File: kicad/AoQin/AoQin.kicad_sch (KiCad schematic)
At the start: 15 parts, among them J1 Conn_02x03_Odd_Even, J10 Conn_02x03_Odd_Even, J11 Conn_02x03_Odd_Even, J12 Conn_02x03_Odd_Even, J14 Screw_Terminal_01x04, J15 Screw_Terminal_01x04, J16 Screw_Terminal_01x04, J2 Conn_02x03_Odd_Even, J3 Screw_Terminal_01x04, J4 Screw_Terminal_01x04, J5 Conn_02x03_Odd_Even, J6 Screw_Terminal_01x04, J8 Screw_Terminal_01x03, J9 Screw_Terminal_01x03

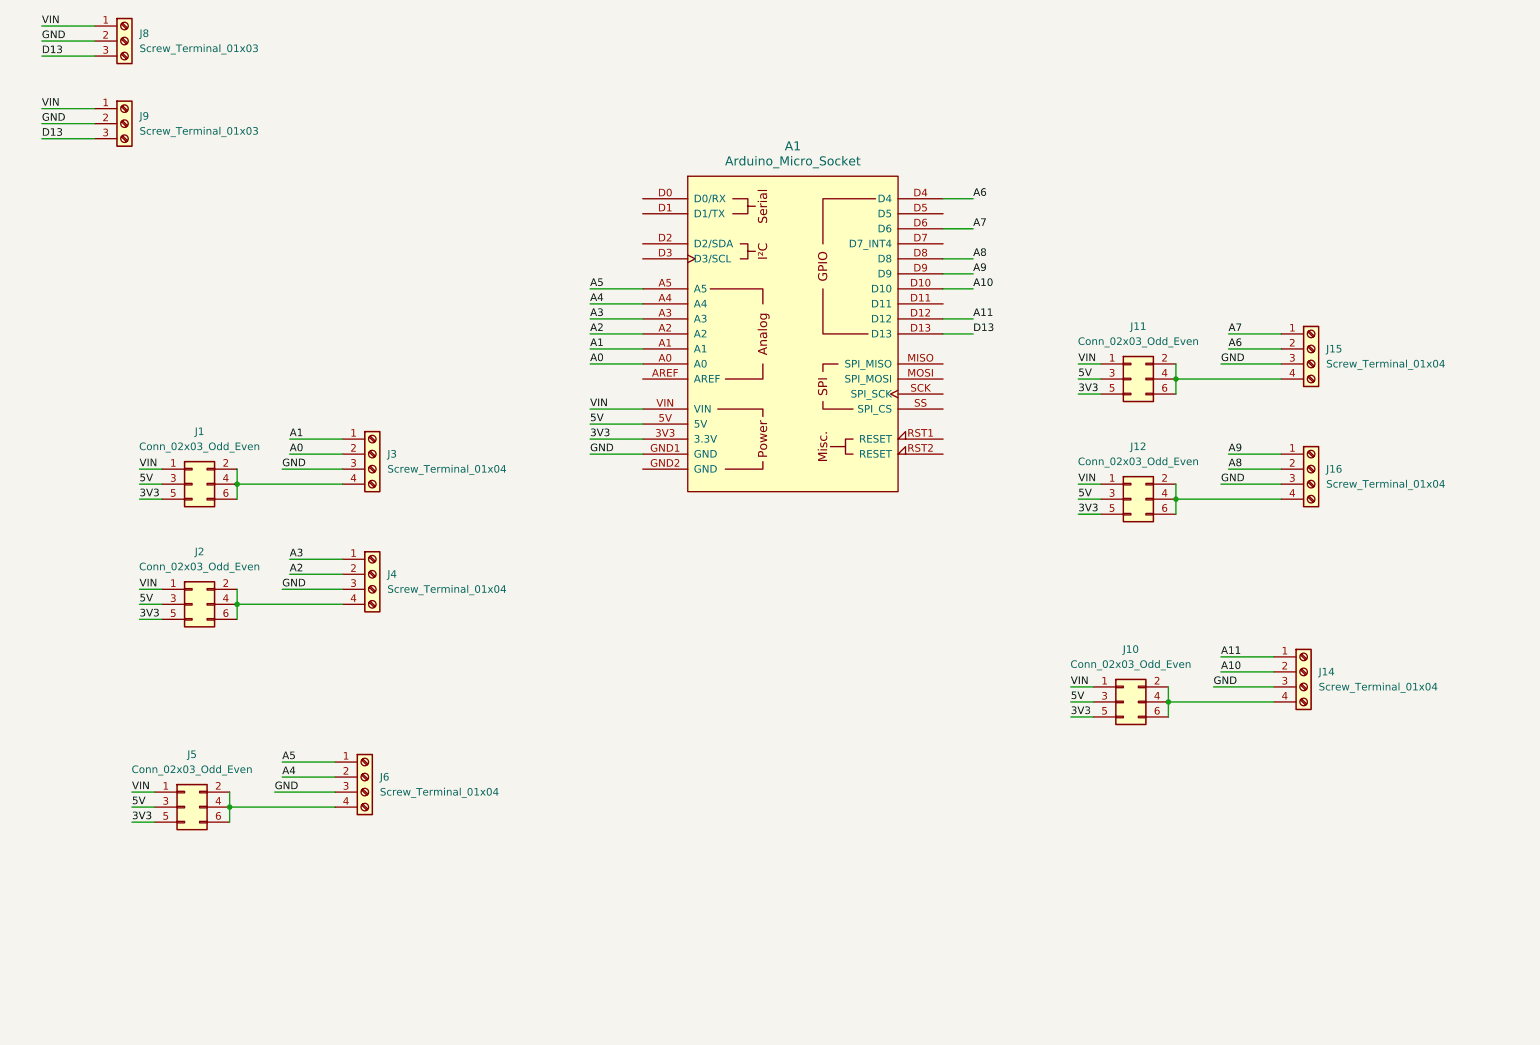
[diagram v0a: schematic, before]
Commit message: The Cave of Echoes
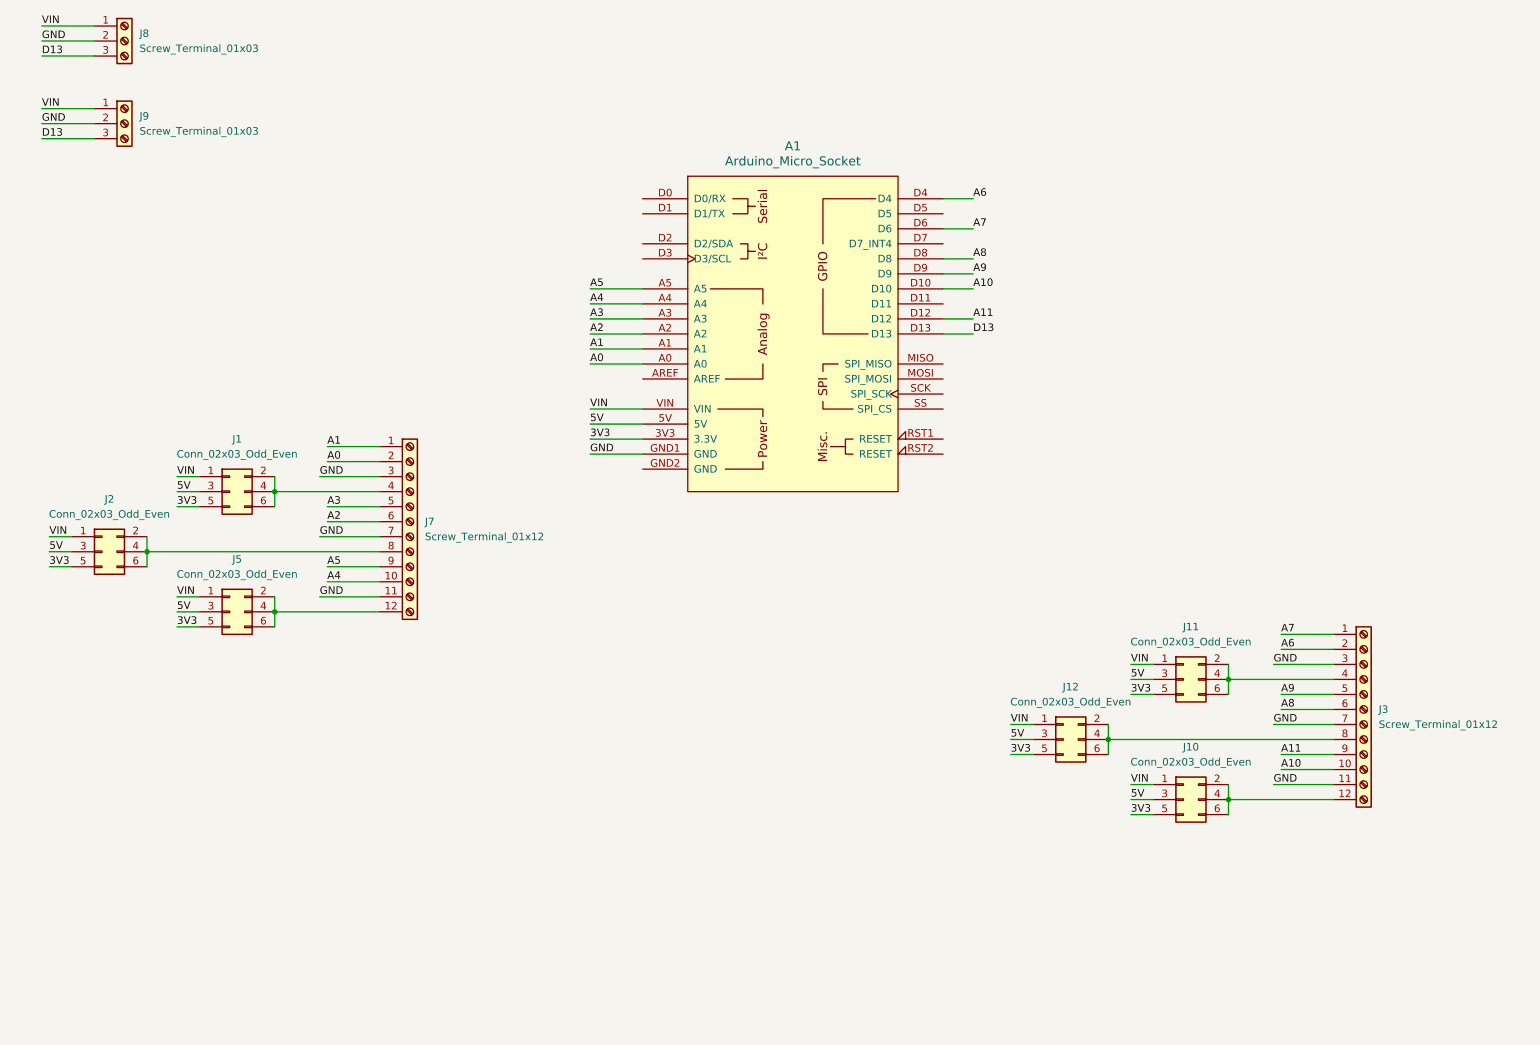
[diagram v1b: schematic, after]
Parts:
- removed J14, J15, J16, J3, J4, J6: Screw_Terminal_01x04, TerminalBlock_Phoenix:TerminalBlock_Phoenix_MKDS-1,5-4-5.08_1x04_P5.08mm_Horizontal, symbol Connector:Screw_Terminal_01x04
- added J3, J7: Screw_Terminal_01x12, footprints:1869318, symbol Connector:Screw_Terminal_01x12
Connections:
- net A0: now also J7.2 (Pin_2)
- net A1: now also J7.1 (Pin_1)
- net A10: now also J3.10 (Pin_10)
- net A11: now also J3.9 (Pin_9)
- net A2: now also J7.6 (Pin_6)
- net A3: now also J7.5 (Pin_5)
- net A4: now also J7.10 (Pin_10)
- net A5: now also J7.9 (Pin_9)
- net A6: now also J3.2 (Pin_2)
- net A7: now also J3.1 (Pin_1)
- net A8: now also J3.6 (Pin_6)
- net A9: now also J3.5 (Pin_5)
- net GND: now also J3.11 (Pin_11), J3.3 (Pin_3), J3.7 (Pin_7), J7.11 (Pin_11), J7.3 (Pin_3), J7.7 (Pin_7)
- net at J11.2 (Pin_2), J11.4 (Pin_4), J11.6 (Pin_6): now also J3.4 (Pin_4)
- net at J10.2 (Pin_2), J10.4 (Pin_4), J10.6 (Pin_6): now also J3.12 (Pin_12)
- net at J2.2 (Pin_2), J2.4 (Pin_4), J2.6 (Pin_6): now also J7.8 (Pin_8)
- net at J5.2 (Pin_2), J5.4 (Pin_4), J5.6 (Pin_6): now also J7.12 (Pin_12)
- net at J12.2 (Pin_2), J12.4 (Pin_4), J12.6 (Pin_6): now also J3.8 (Pin_8)
- net at J1.2 (Pin_2), J1.4 (Pin_4), J1.6 (Pin_6): now also J7.4 (Pin_4)
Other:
- moved on the sheet: J1, J10, J11, J12, J2, J5

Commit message: The Sword of Veracity
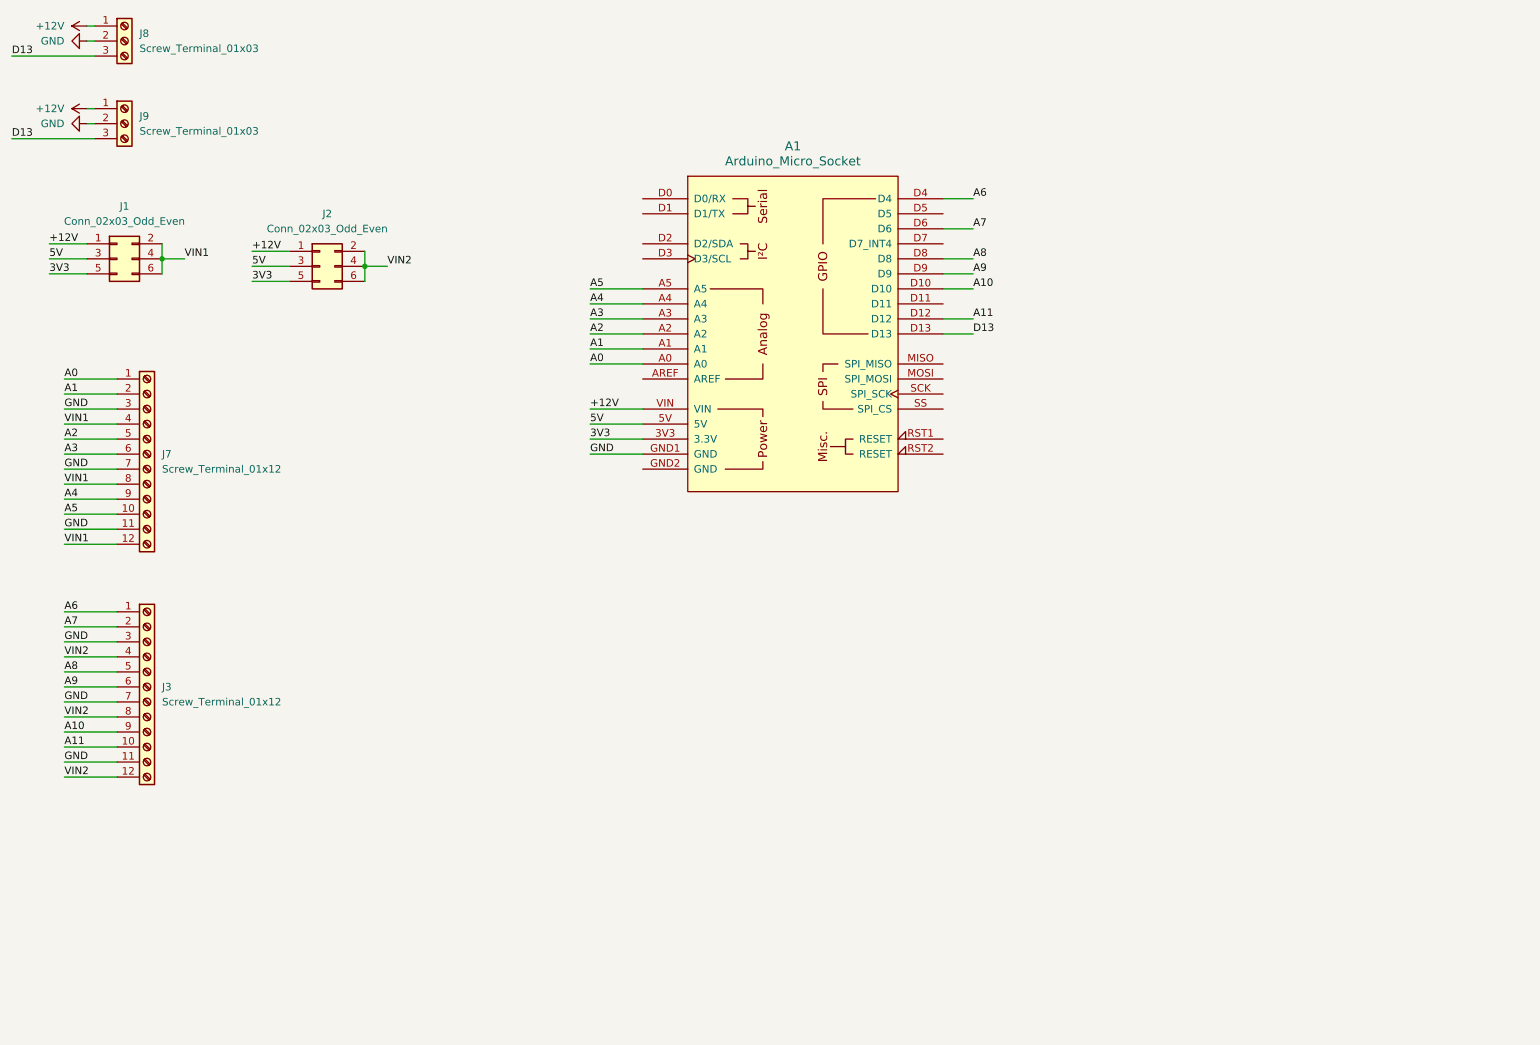
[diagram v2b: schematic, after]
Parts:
- removed J10, J11, J12, J5: Conn_02x03_Odd_Even, Connector_PinHeader_2.54mm:PinHeader_2x03_P2.54mm_Vertical, symbol Connector_Generic:Conn_02x03_Odd_Even
- J3, J7: MPN (none) -> MKDSN 1.5/12
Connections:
- net A0: now also J7.1 (Pin_1); no longer J7.2 (Pin_2)
- net A1: now also J7.2 (Pin_2); no longer J7.1 (Pin_1)
- net A10: now also J3.9 (Pin_9); no longer J3.10 (Pin_10)
- net A11: now also J3.10 (Pin_10); no longer J3.9 (Pin_9)
- net A2: now also J7.5 (Pin_5); no longer J7.6 (Pin_6)
- net A3: now also J7.6 (Pin_6); no longer J7.5 (Pin_5)
- net A4: now also J7.9 (Pin_9); no longer J7.10 (Pin_10)
- net A5: now also J7.10 (Pin_10); no longer J7.9 (Pin_9)
- net A6: now also J3.1 (Pin_1); no longer J3.2 (Pin_2)
- net A7: now also J3.2 (Pin_2); no longer J3.1 (Pin_1)
- net A8: now also J3.5 (Pin_5); no longer J3.6 (Pin_6)
- net A9: now also J3.6 (Pin_6); no longer J3.5 (Pin_5)
- net VIN2: now reaches J3.4 (Pin_4)
- net VIN2: now also J2.2 (Pin_2), J2.4 (Pin_4), J2.6 (Pin_6), J3.12 (Pin_12), J3.8 (Pin_8)
- net VIN1: now reaches J7.12 (Pin_12)
- net VIN1: now also J1.2 (Pin_2), J1.4 (Pin_4), J1.6 (Pin_6), J7.4 (Pin_4), J7.8 (Pin_8)
- net VIN renamed +12V
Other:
- moved on the sheet: J3, J7

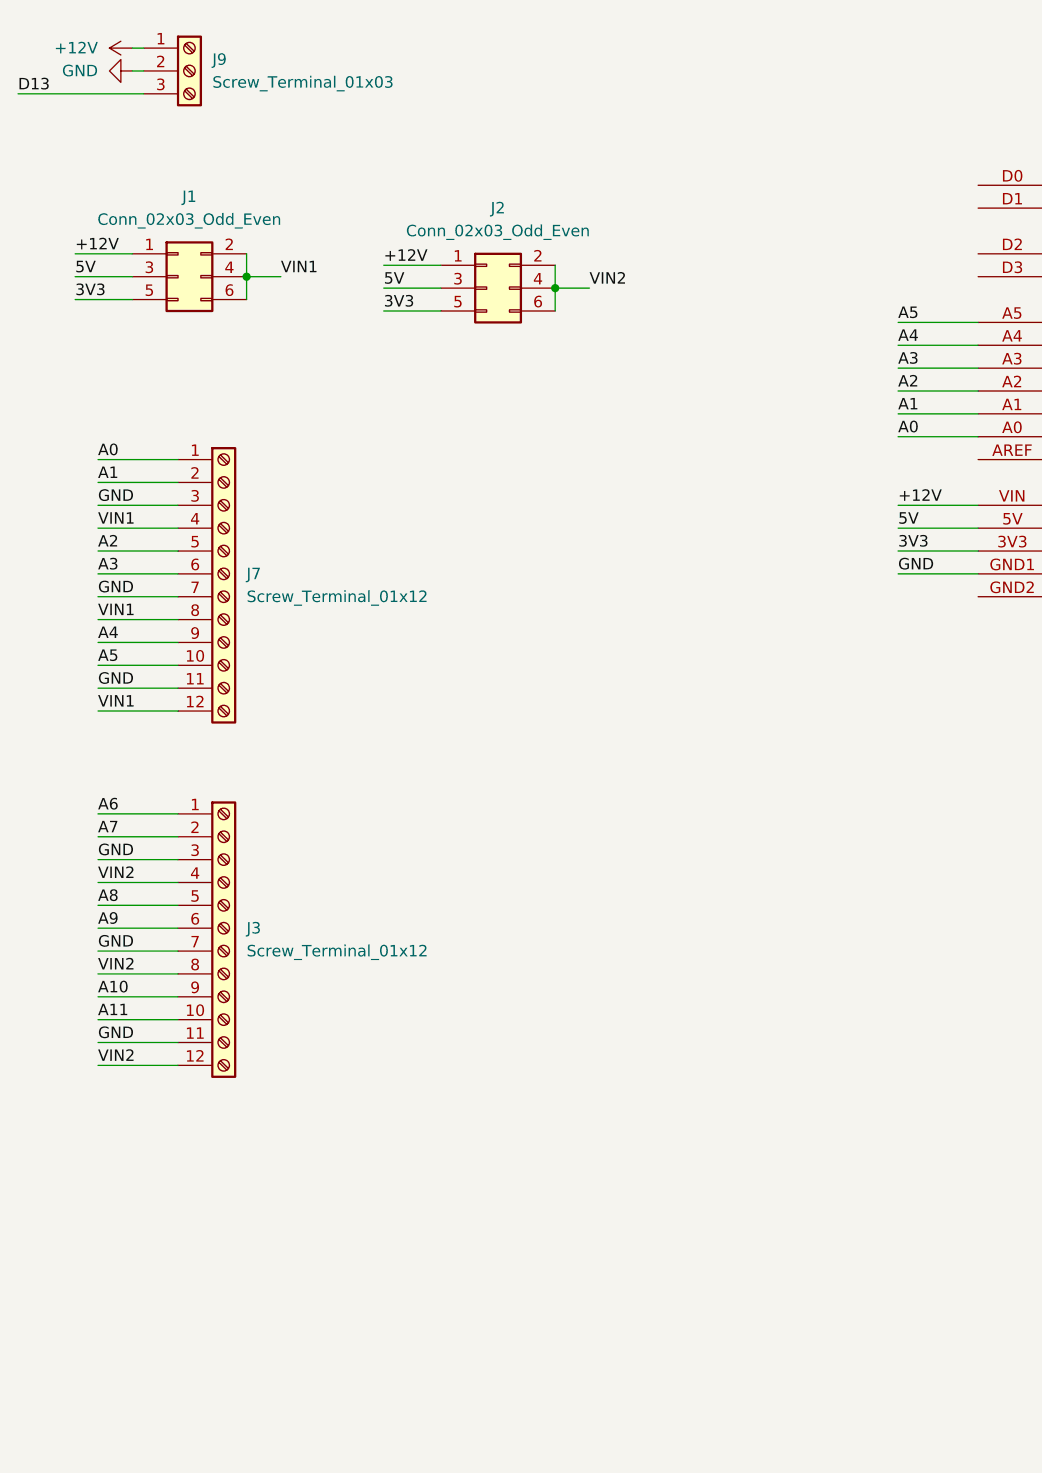
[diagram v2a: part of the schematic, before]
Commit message: When a Man Loves a Woman
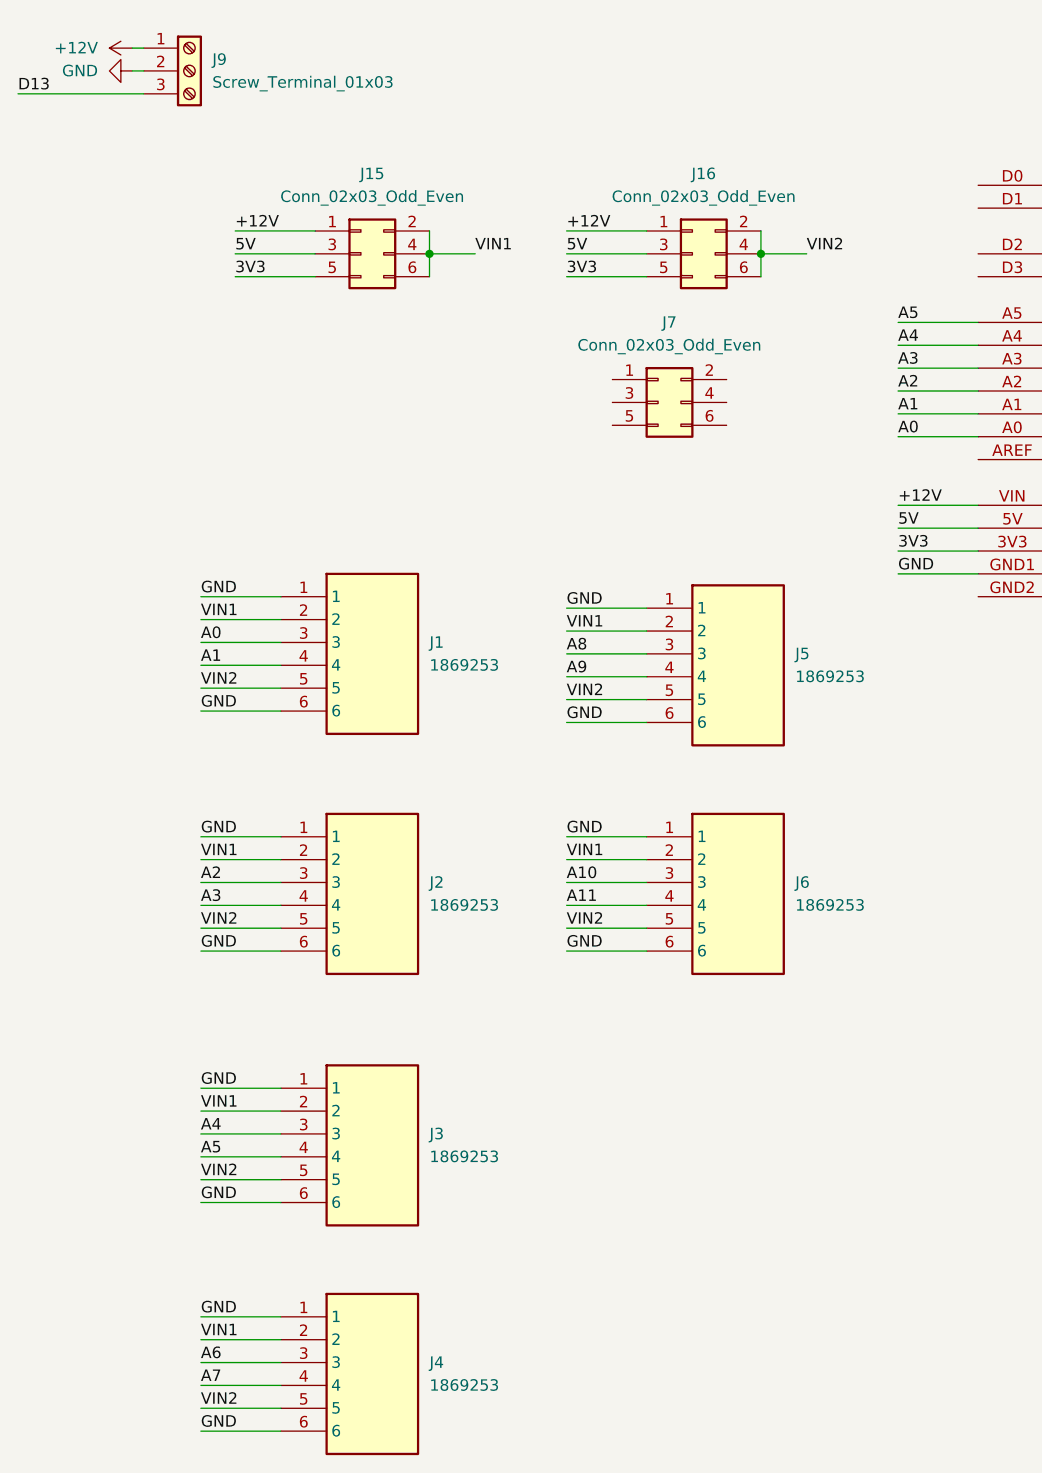
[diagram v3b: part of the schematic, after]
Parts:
- removed J1, J2: Conn_02x03_Odd_Even, Connector_PinHeader_2.54mm:PinHeader_2x03_P2.54mm_Vertical, symbol Connector_Generic:Conn_02x03_Odd_Even
- removed J3, J7: Screw_Terminal_01x12, footprints:1869318, symbol Connector:Screw_Terminal_01x12
- added J1, J2, J3, J4, J5, J6: 1869253, footprints:SMKDSN_15_6_508, symbol PheonixContact:1869253
- added J15, J16, J7: Conn_02x03_Odd_Even, Connector_PinHeader_2.54mm:PinHeader_2x03_P2.54mm_Vertical, symbol Connector_Generic:Conn_02x03_Odd_Even
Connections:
- net +12V: now also J15.1 (Pin_1), J16.1 (Pin_1)
- net 3V3: now also J15.5 (Pin_5), J16.5 (Pin_5)
- net 5V: now also J15.3 (Pin_3), J16.3 (Pin_3)
- net A0: now also J1.3
- net A1: now also J1.4
- net A10: now also J6.3
- net A11: now also J6.4
- net A2: now also J2.3
- net A3: now also J2.4
- net A4: now also J3.3
- net A5: now also J3.4
- net A6: now also J4.3
- net A7: now also J4.4
- net A8: now also J5.3
- net A9: now also J5.4
- net GND: now also J1.1, J1.6, J2.1, J2.6, J3.1, J3.6, J4.1, J4.6, J5.1, J5.6, J6.1, J6.6
- net VIN1: now also J1.2, J15.2 (Pin_2), J15.4 (Pin_4), J15.6 (Pin_6), J2.2, J3.2, J4.2, J5.2, J6.2
- net VIN2: now also J1.5, J16.2 (Pin_2), J16.4 (Pin_4), J16.6 (Pin_6), J2.5, J3.5, J4.5, J5.5, J6.5
